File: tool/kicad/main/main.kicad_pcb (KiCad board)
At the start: 2 copper layers, 81.7 x 45 mm, 115 parts, among them J1 MICRO-USB-AB, K1 CONN_3, P1 TEST_POINT, P10 TEST_POINT, P11 TEST_POINT, P12 TEST_POINT, P13 TEST_POINT, P14 TEST_POINT, P15 TEST_POINT, P16 TEST_POINT, P17 TEST_POINT, P18 TEST_POINT, P19 TEST_POINT, P2 TEST_POINT, P20 TEST_POINT, P21 TEST_POINT, P22 TEST_POINT, P23 TEST_POINT, P24 TEST_POINT, P25 TEST_POINT, P26 TEST_POINT, P27 TEST_POINT, P28 TEST_POINT, P29 TEST_POINT, P3 TEST_POINT, P30 CONN_3X2, P31 CONN_7, P35 CONN_6, P37 TEST_POINT, P38 TEST_POINT, P4 TEST_POINT, P5 CONN_6, P6 TEST_POINT, P7 TEST_POINT, P8 TEST_POINT, P9 TEST_POINT, U1 SN74LVC2T45, U2 ST-USBLC6-2, U3 EFM32GG332, U4 YM2413, X1 48Mhz, X2 CRYSTAL

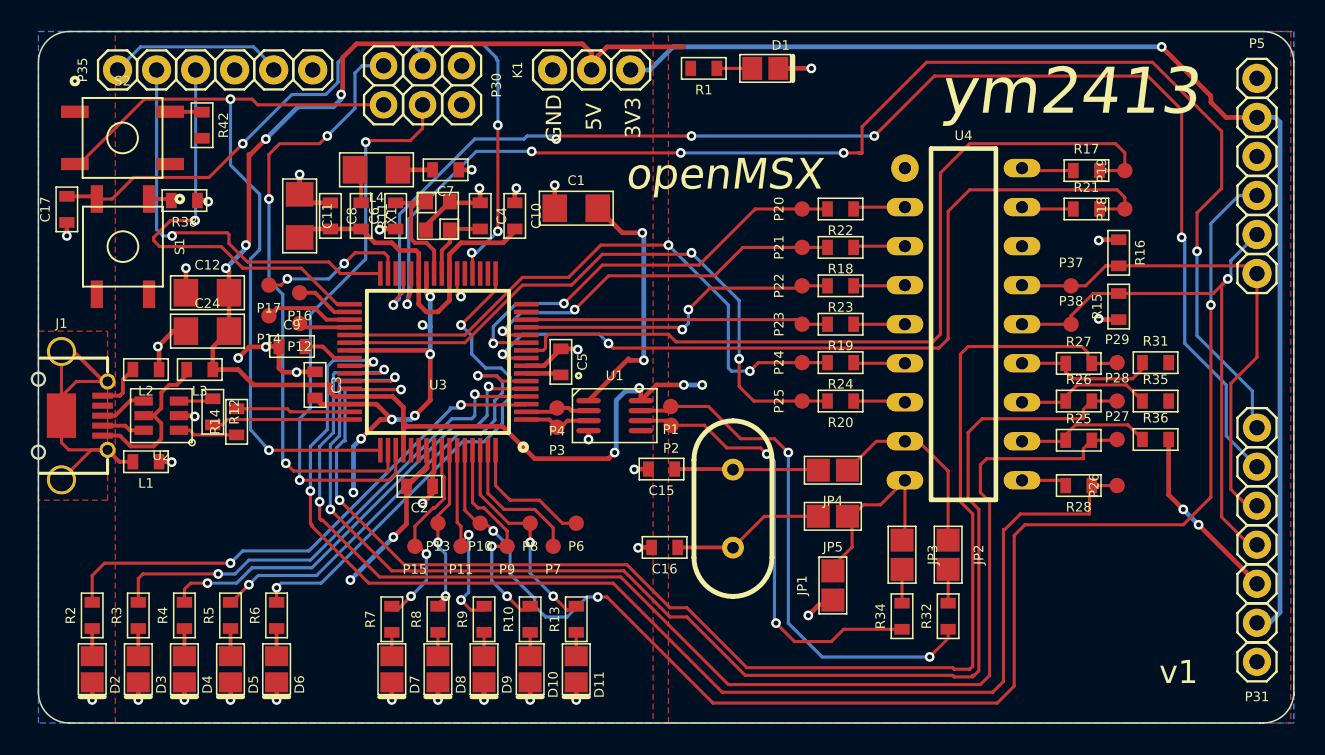
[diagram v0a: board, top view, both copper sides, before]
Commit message: main board WIP
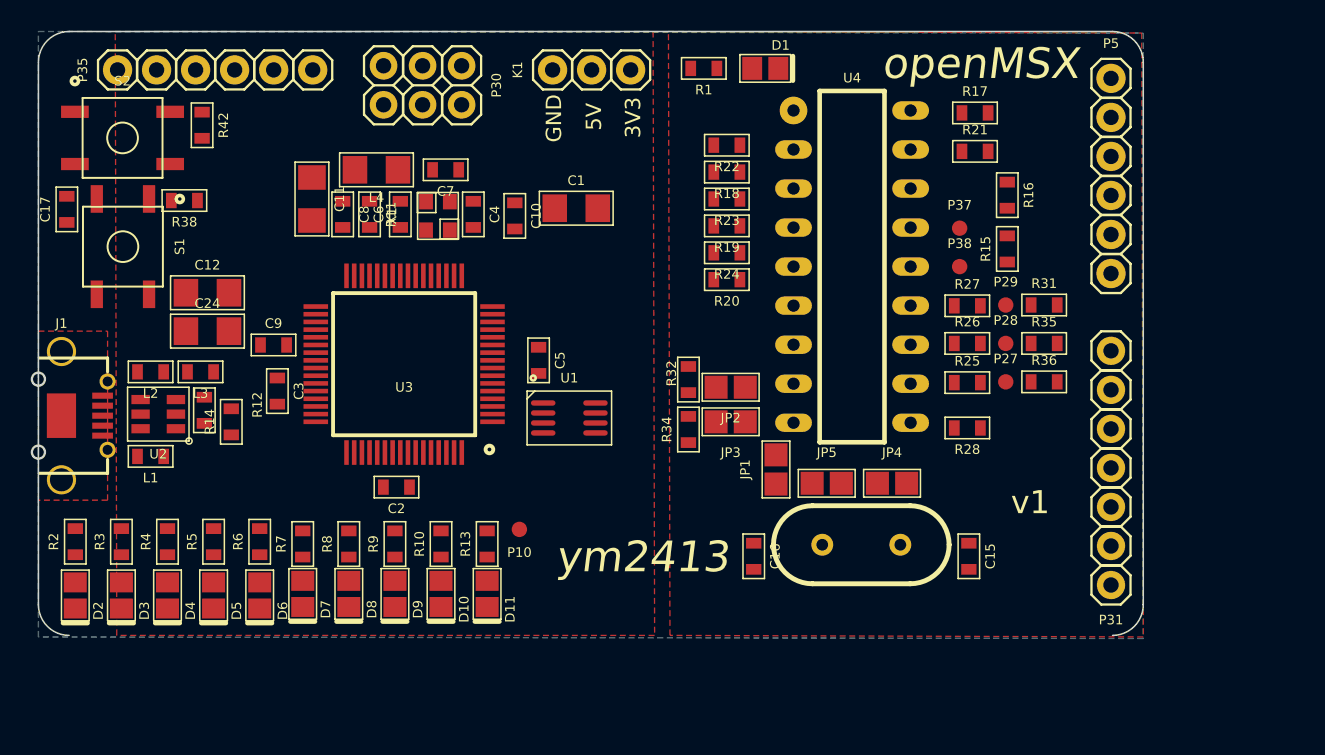
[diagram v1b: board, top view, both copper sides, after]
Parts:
- removed P1, P11, P12, P13, P14, P15, P16, P17, P18, P19, P2, P20, P21, P22, P23, P24, P25, P26, P3, P4, P6, P7, P8, P9: TEST_POINT, pretty:Test_Pad_1mm
- moved R32 22.9 mm to (126.5, 96.2), turned to 270 degrees
- moved C15 20.8 mm to (144.8, 107.8), turned to 270 degrees
- moved R34 18.5 mm to (126.5, 99.5)
- moved JP2 17.9 mm to (129.2, 96.8), turned to 180 degrees
- moved JP3 14.1 mm to (129.2, 99.0), turned to 180 degrees
- moved R20 10.8 mm to (129.0, 89.8)
- moved P31 10.7 mm to (154.0, 102.0)
- moved R24 10.3 mm to (129.0, 88.0)
- moved R19 9.78 mm to (129.0, 86.2)
- moved P5 9.50 mm to (154.0, 83.0)
- moved R23 9.31 mm to (129.0, 84.5)
- moved R18 8.88 mm to (129.0, 82.8)
- moved X2 8.67 mm to (137.8, 107.0), turned to 0 degrees
- moved R22 8.48 mm to (129.0, 81.0)
- moved JP1 8.41 mm to (132.2, 102.1)
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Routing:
- net +3.3V: track 140.2 -> 0.00 mm, vias 12 -> 0
- net +5V: track 105.7 -> 0.00 mm, vias 10 -> 0
- net /MIDI_IN: track 92.9 -> 0.00 mm, vias 3 -> 0
- net /~IC: track 92.2 -> 0.00 mm, vias 2 -> 0
- net /RO_SAMPLE: track 89.4 -> 0.00 mm, vias 5 -> 0
- net /MO_SAMPLE: track 89.3 -> 0.00 mm, vias 5 -> 0
- net /~CS: track 89.1 -> 0.00 mm, vias 2 -> 0
- net /~WE: track 87.9 -> 0.00 mm, vias 2 -> 0
- net /A0: track 85.0 -> 0.00 mm, vias 2 -> 0
- net /D0: track 54.8 -> 0.00 mm, vias 2 -> 0
- net /D1: track 54.5 -> 0.00 mm
- net GND: track 54.0 -> 0.00 mm, vias 35 -> 0
- net /SWC: track 53.6 -> 0.00 mm, vias 2 -> 0
- net /~RESET: track 50.5 -> 0.00 mm, vias 4 -> 0
- net /D7: track 40.8 -> 0.00 mm, vias 2 -> 0
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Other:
- board size 81.7 x 45 mm -> 71.9 x 39.3 mm
